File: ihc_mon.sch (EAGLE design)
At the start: 36 parts, among them IC1 PIC18F1220P, IC3 ADM3095EBRZ, X1 22-23-2021, X2 22-23-2021

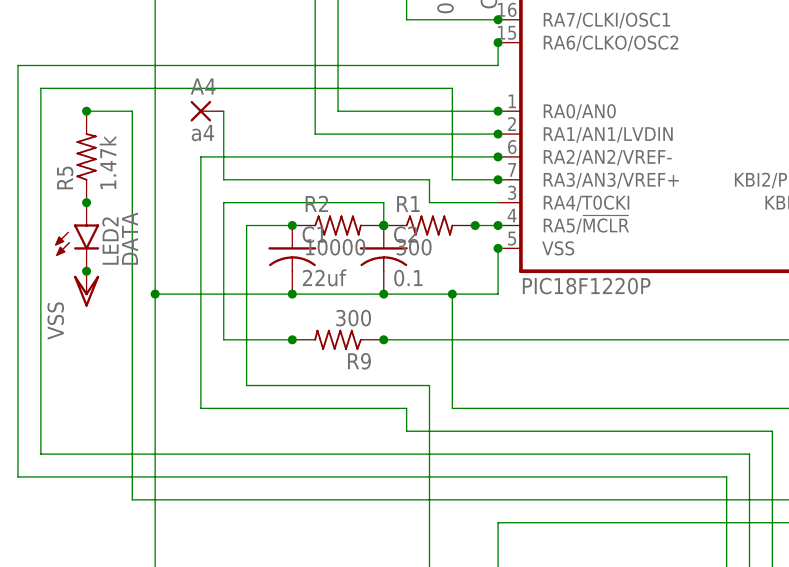
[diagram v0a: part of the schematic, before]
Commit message: up
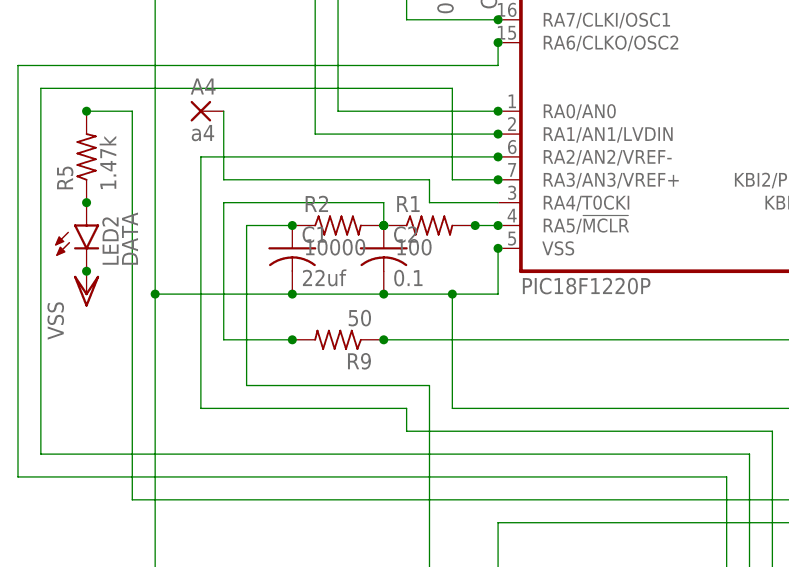
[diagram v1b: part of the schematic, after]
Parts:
- R1: value 300 -> 100
- R9: value 300 -> 50
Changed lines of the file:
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@@
 <part name="C3" library="rcl" library_urn="urn:adsk.eagle:library:334" deviceset="C-US" device="C0805" package3d_urn="urn:adsk.eagle:package:23617/2" value="0.1"/>
 <part name="C7" library="rcl" library_urn="urn:adsk.eagle:library:334" deviceset="C-US" device="C0805" package3d_urn="urn:adsk.eagle:package:23617/2" value="22uf"/>
-<part name="R1" library="rcl" library_urn="urn:adsk.eagle:library:334" deviceset="R-US_" device="R0805" package3d_urn="urn:adsk.eagle:package:23553/2" value="300"/>
+<part name="R1" library="rcl" library_urn="urn:adsk.eagle:library:334" deviceset="R-US_" device="R0805" package3d_urn="urn:adsk.eagle:package:23553/2" value="100"/>
 <part name="R2" library="rcl" library_urn="urn:adsk.eagle:library:334" deviceset="R-US_" device="R0805" package3d_urn="urn:adsk.eagle:package:23553/2" value="10000"/>
 <part name="IC3" library="SamacSys_Parts" deviceset="ADM3095EBRZ" device=""/>
@@
 <part name="LED1" library="led" library_urn="urn:adsk.eagle:library:259" deviceset="LED" device="CHIPLED_1206" package3d_urn="urn:adsk.eagle:package:15823/2" value="POWER"/>
 <part name="VSS18" library="supply1" deviceset="VSS" device=""/>
-<part name="R9" library="rcl" library_urn="urn:adsk.eagle:library:334" deviceset="R-US_" device="R0805" package3d_urn="urn:adsk.eagle:package:23553/2" value="300"/>
+<part name="R9" library="rcl" library_urn="urn:adsk.eagle:library:334" deviceset="R-US_" device="R0805" package3d_urn="urn:adsk.eagle:package:23553/2" value="50"/>
 </parts>
 <sheets>

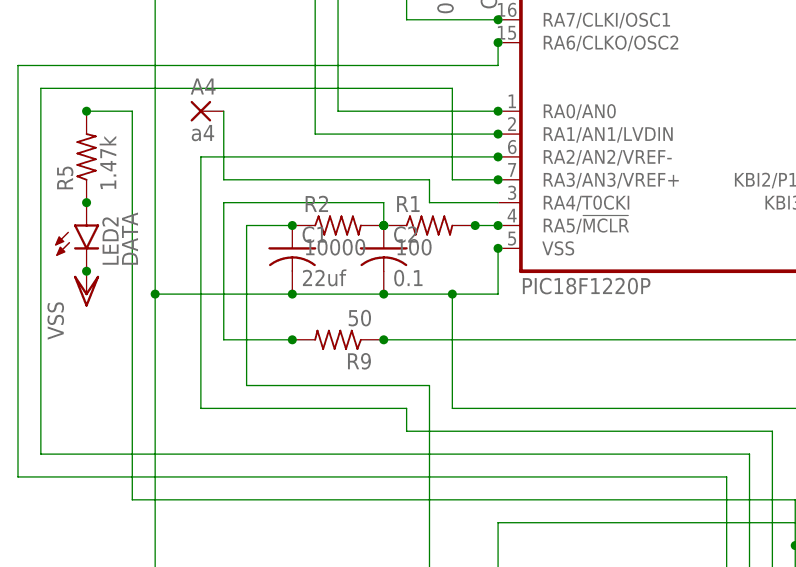
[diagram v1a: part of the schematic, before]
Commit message: up
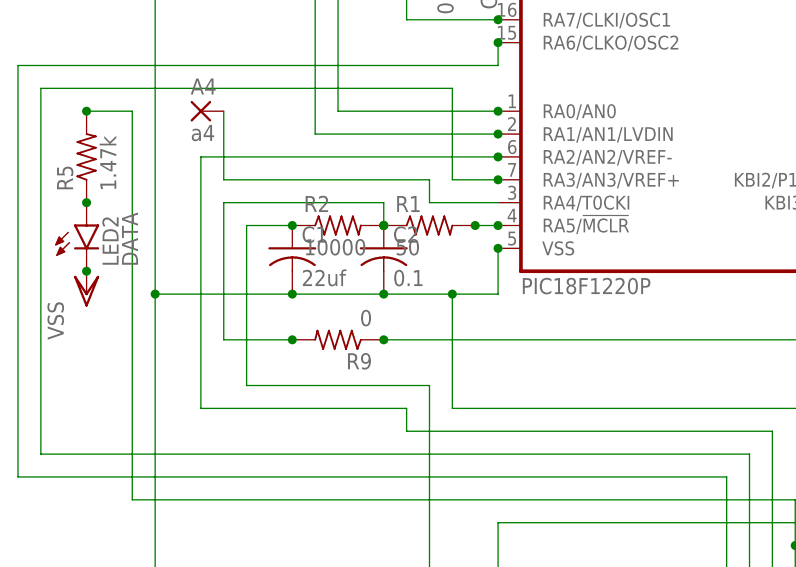
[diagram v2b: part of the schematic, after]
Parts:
- R1: value 100 -> 50
- R9: value 50 -> 0
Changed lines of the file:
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@@
 <part name="C3" library="rcl" library_urn="urn:adsk.eagle:library:334" deviceset="C-US" device="C0805" package3d_urn="urn:adsk.eagle:package:23617/2" value="0.1"/>
 <part name="C7" library="rcl" library_urn="urn:adsk.eagle:library:334" deviceset="C-US" device="C0805" package3d_urn="urn:adsk.eagle:package:23617/2" value="22uf"/>
-<part name="R1" library="rcl" library_urn="urn:adsk.eagle:library:334" deviceset="R-US_" device="R0805" package3d_urn="urn:adsk.eagle:package:23553/2" value="100"/>
+<part name="R1" library="rcl" library_urn="urn:adsk.eagle:library:334" deviceset="R-US_" device="R0805" package3d_urn="urn:adsk.eagle:package:23553/2" value="50"/>
 <part name="R2" library="rcl" library_urn="urn:adsk.eagle:library:334" deviceset="R-US_" device="R0805" package3d_urn="urn:adsk.eagle:package:23553/2" value="10000"/>
 <part name="IC3" library="SamacSys_Parts" deviceset="ADM3095EBRZ" device=""/>
@@
 <part name="LED1" library="led" library_urn="urn:adsk.eagle:library:259" deviceset="LED" device="CHIPLED_1206" package3d_urn="urn:adsk.eagle:package:15823/2" value="POWER"/>
 <part name="VSS18" library="supply1" deviceset="VSS" device=""/>
-<part name="R9" library="rcl" library_urn="urn:adsk.eagle:library:334" deviceset="R-US_" device="R0805" package3d_urn="urn:adsk.eagle:package:23553/2" value="50"/>
+<part name="R9" library="rcl" library_urn="urn:adsk.eagle:library:334" deviceset="R-US_" device="R0805" package3d_urn="urn:adsk.eagle:package:23553/2" value="0"/>
 </parts>
 <sheets>
